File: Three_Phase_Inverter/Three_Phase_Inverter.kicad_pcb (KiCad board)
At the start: 2 copper layers, 62.5 x 123 mm, 53 parts, among them J3 3 phase output, J5 POWER, J6 OLED Display pins, Q1 IRLZ44N, Q2 IRLZ44N, Q3 IRLZ44N, Q4 IRLZ44N, Q5 IRLZ44N, Q6 IRLZ44N, U1 L7805, U2 PC817, U3 PC817, U4 PC817, U5 PC817, U6 PC817, U7 PC817, U8 ESP32-WROOM-32

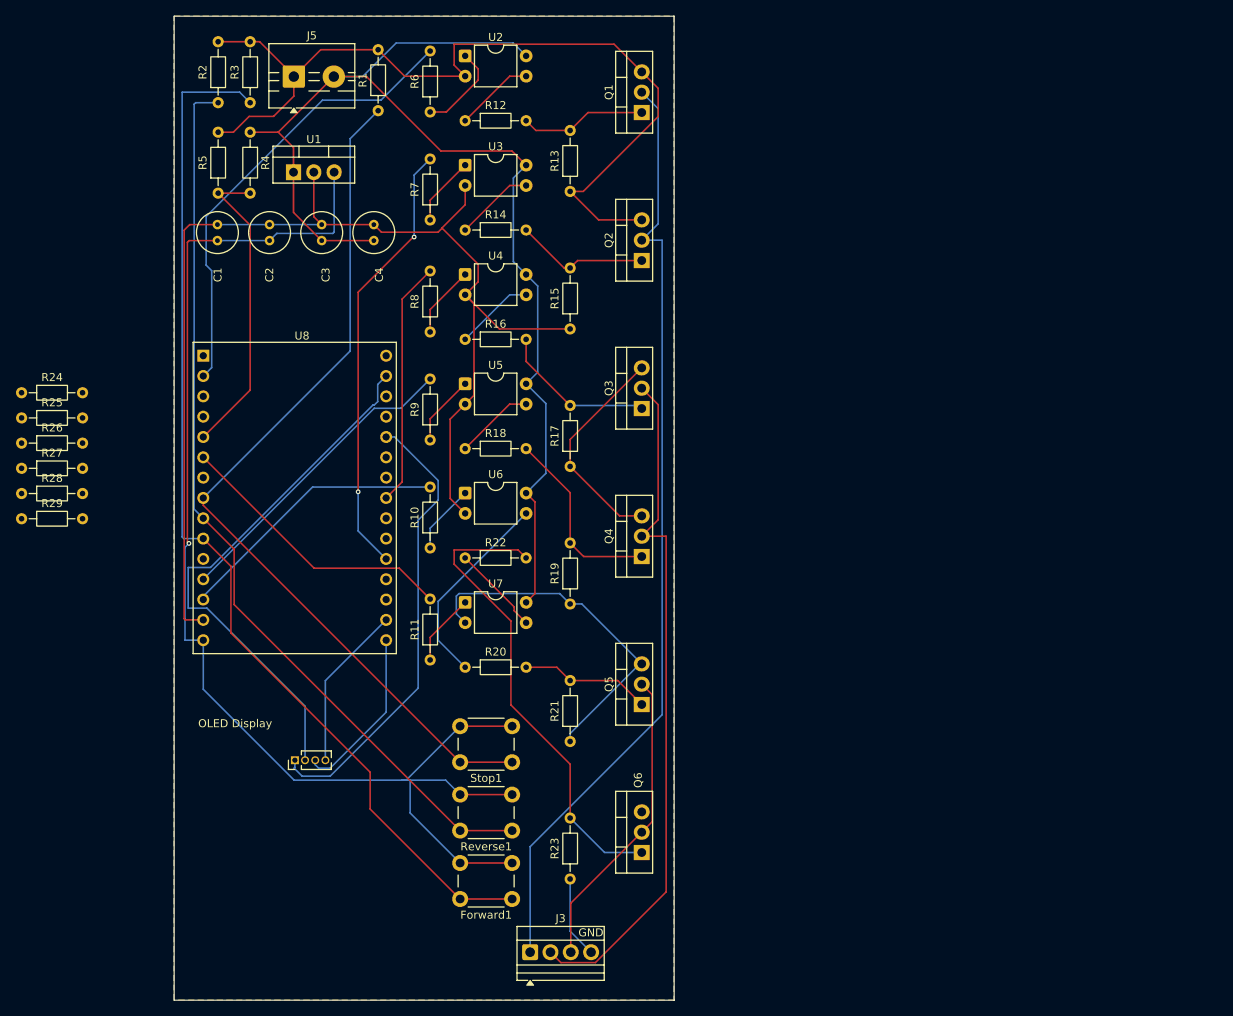
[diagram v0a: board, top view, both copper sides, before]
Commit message: changes
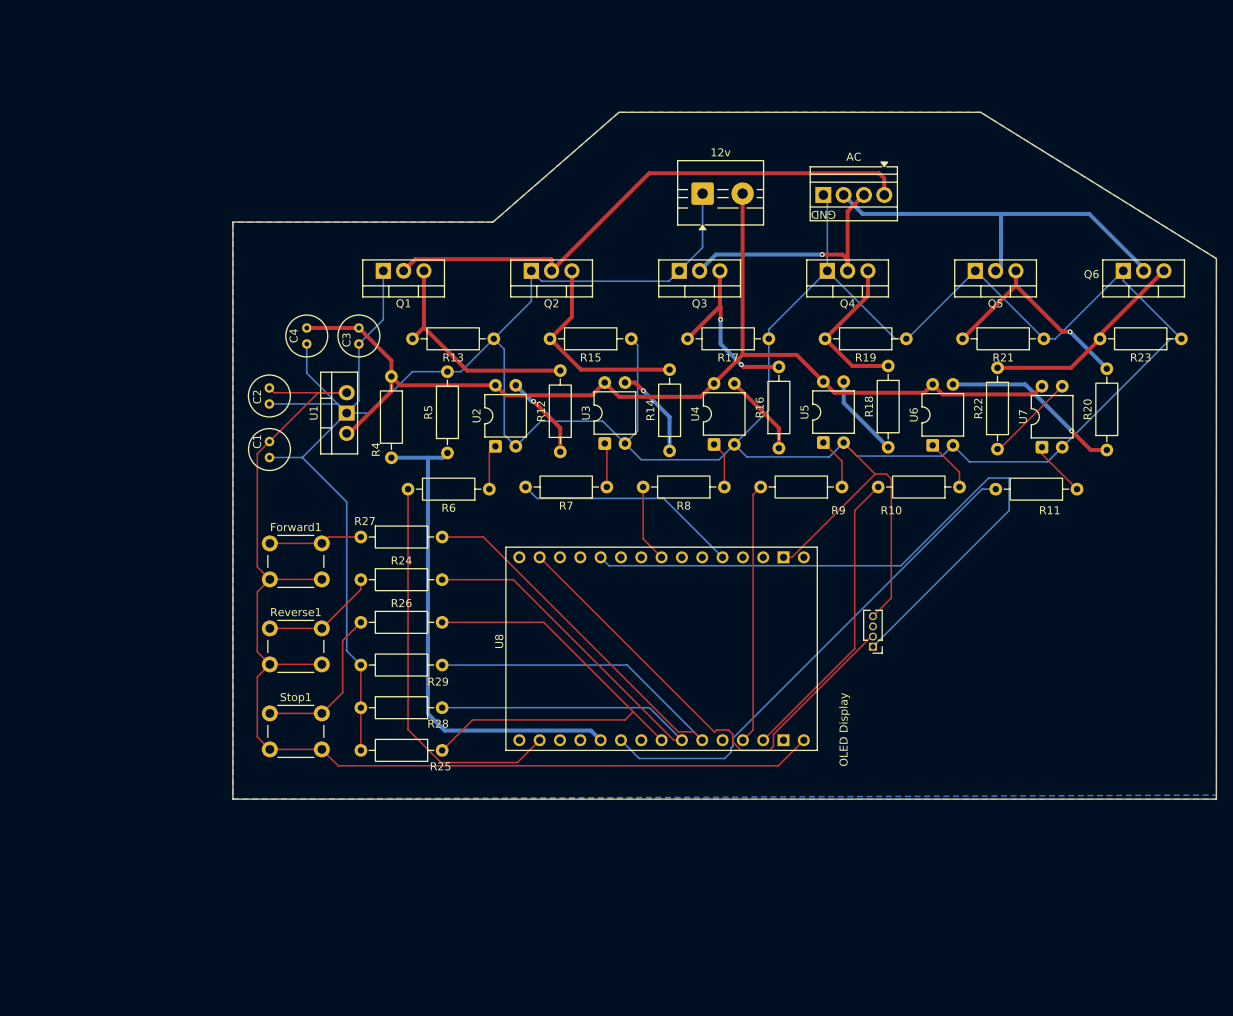
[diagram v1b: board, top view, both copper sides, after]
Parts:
- removed R1, R2, R3: 1k, Resistor_THT:R_Axial_DIN0204_L3.6mm_D1.6mm_P7.62mm_Horizontal
- R10, R11, R12, R13, R14, R15, R16, R17, R18, R19, R20, R21, R22, R23, R24, R25, R26, R27, R28, R29, R4, R5, R6, R7, R8, R9: footprint Resistor_THT:R_Axial_DIN0204_L3.6mm_D1.6mm_P7.62mm_Horizontal -> Resistor_THT:R_Axial_DIN0207_L6.3mm_D2.5mm_P10.16mm_Horizontal
- moved AC 104.5 mm to (198.8, 74.8), turned to 180 degrees
- moved R23 102.0 mm to (235.9, 92.8), turned to 180 degrees
- moved Q6 97.7 mm to (233.7, 84.3), turned to 180 degrees
- moved R20 84.7 mm to (226.6, 106.7), turned to 90 degrees
- moved R11 83.6 mm to (222.9, 111.6), turned to 180 degrees
- moved R21 77.7 mm to (218.7, 92.8), turned to 180 degrees
- moved U7 74.7 mm to (218.5, 106.4), turned to 90 degrees
- moved J6 73.6 mm to (197.3, 131.3), turned to 180 degrees
- moved Q5 71.6 mm to (215.2, 84.3), turned to 180 degrees
- moved R22 67.9 mm to (212.9, 106.6), turned to 90 degrees
- moved R25 67.0 mm to (143.5, 144.3), turned to 180 degrees
- moved R10 66.6 mm to (208.2, 111.4), turned to 180 degrees
- moved U8 62.2 mm to (153.2, 143.0), turned to 90 degrees
- moved R28 59.0 mm to (143.5, 138.9), turned to 180 degrees
- moved U6 58.7 mm to (204.8, 106.1), turned to 90 degrees
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- renumbered J5 to 12v, J3 to AC
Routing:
- net GPIO33: track 114.2 -> 0.00 mm
- net GPIO32*: track 146.0 -> 62.6 mm
- net GPIO27: track 0.00 -> 79.4 mm
- net GPIO25: track 132.2 -> 59.4 mm
- net GPIO26: track 0.00 -> 69.9 mm
- net GND: track 366.4 -> 421.5 mm
- net Net-(J3-Pin_2): track 86.4 -> 31.3 mm, vias 0 -> 1
- net Net-(J3-Pin_1): track 118.6 -> 69.5 mm
- net Net-(Q6-G): track 59.7 -> 26.1 mm
- net GPIO4*: track 55.4 -> 28.3 mm, vias 2 -> 0
- net GPIO21(SDA): track 57.3 -> 84.2 mm
- net GPIO35: track 38.6 -> 62.2 mm
- net 3.3V: track 21.5 -> 0.00 mm
- net GPIO5*: track 30.6 -> 9.75 mm
- net Net-(R26-Pad1): track 0.00 -> 19.9 mm
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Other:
- board size 62.5 x 123 mm -> 122.9 x 85.9 mm
